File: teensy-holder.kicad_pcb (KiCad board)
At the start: 2 copper layers, 55 x 60 mm, 20 parts, among them P1 BNC, P2 A1, P3 A2, P4 A1, U1 Teensy3.2_DIP

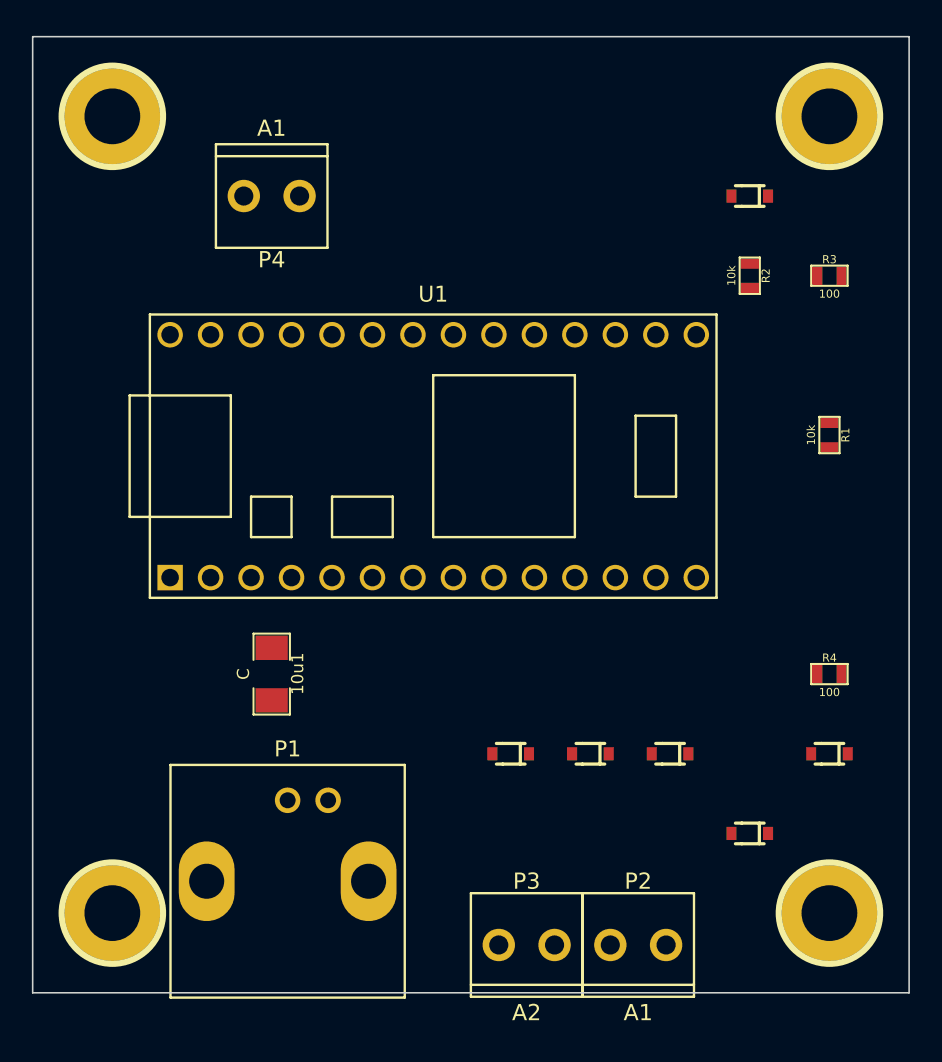
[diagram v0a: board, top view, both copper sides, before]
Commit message: board layout
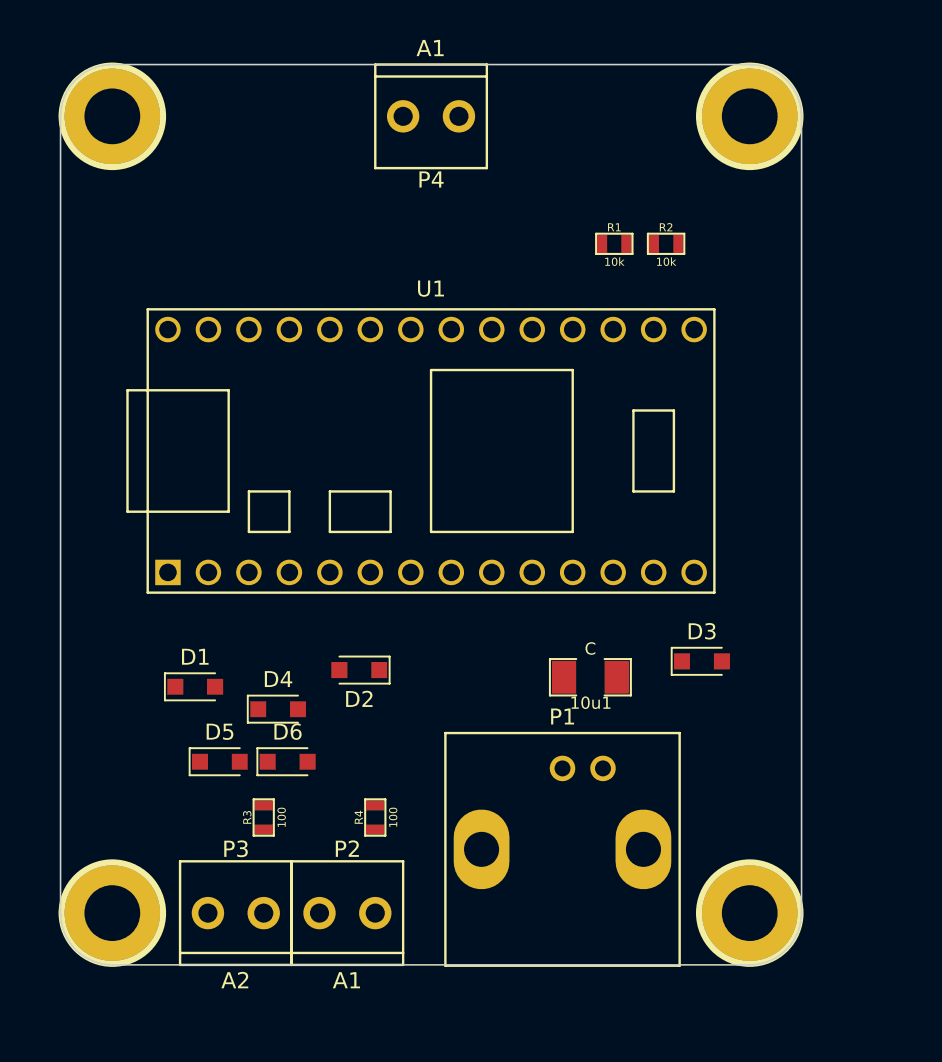
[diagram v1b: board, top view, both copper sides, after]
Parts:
- D1, D2, D3, D4, D5, D6: footprint visgence_parts:SOD-323 -> Diodes_SMD:D_SOD-323_HandSoldering
- moved R3 49.2 mm to (44.5, 84.0), turned to 90 degrees
- moved D1 46.5 mm to (40.2, 75.8)
- moved D2 30.0 mm to (50.5, 74.8), turned to 180 degrees
- moved R4 29.9 mm to (51.5, 84.0), turned to 90 degrees
- moved D4 24.8 mm to (45.4, 77.2)
- moved 10u1 20.0 mm to (65.0, 75.2), turned to 180 degrees
- moved D6 19.0 mm to (46.0, 80.5)
- moved P2 18.4 mm to (49.8, 90.0)
- moved P3 18.4 mm to (42.8, 90.0)
- moved D5 18.3 mm to (41.8, 80.5)
- moved R1 18.1 mm to (66.5, 48.0), turned to 0 degrees
- moved P1 17.4 mm to (63.2, 86.0)
- moved D3 11.2 mm to (72.0, 74.2)
- moved P4 11.2 mm to (55.0, 40.0)
- moved R2 5.62 mm to (69.8, 48.0), turned to 0 degrees
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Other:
- board size 55 x 60 mm -> 46.5 x 56.5 mm
